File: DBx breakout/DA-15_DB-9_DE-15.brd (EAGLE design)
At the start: 19.1 x 38.1 mm, 3 parts

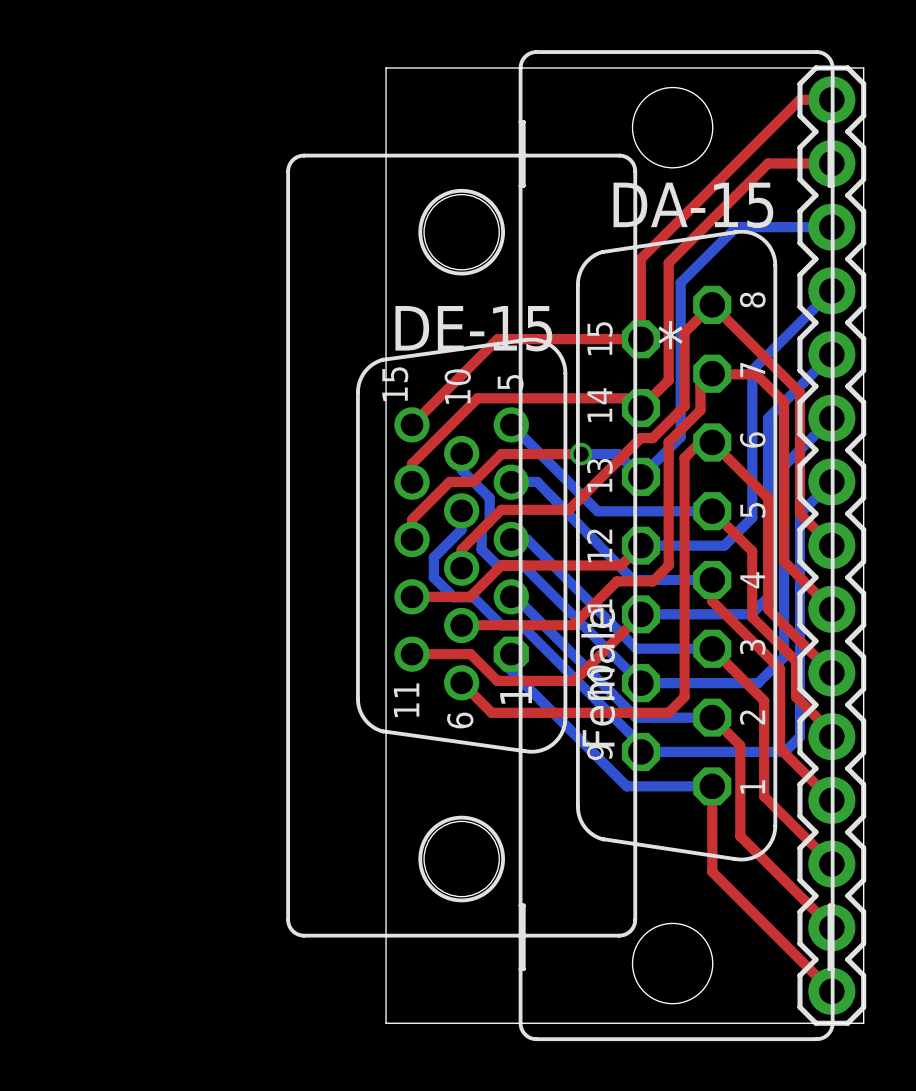
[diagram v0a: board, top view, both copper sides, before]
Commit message: updated board
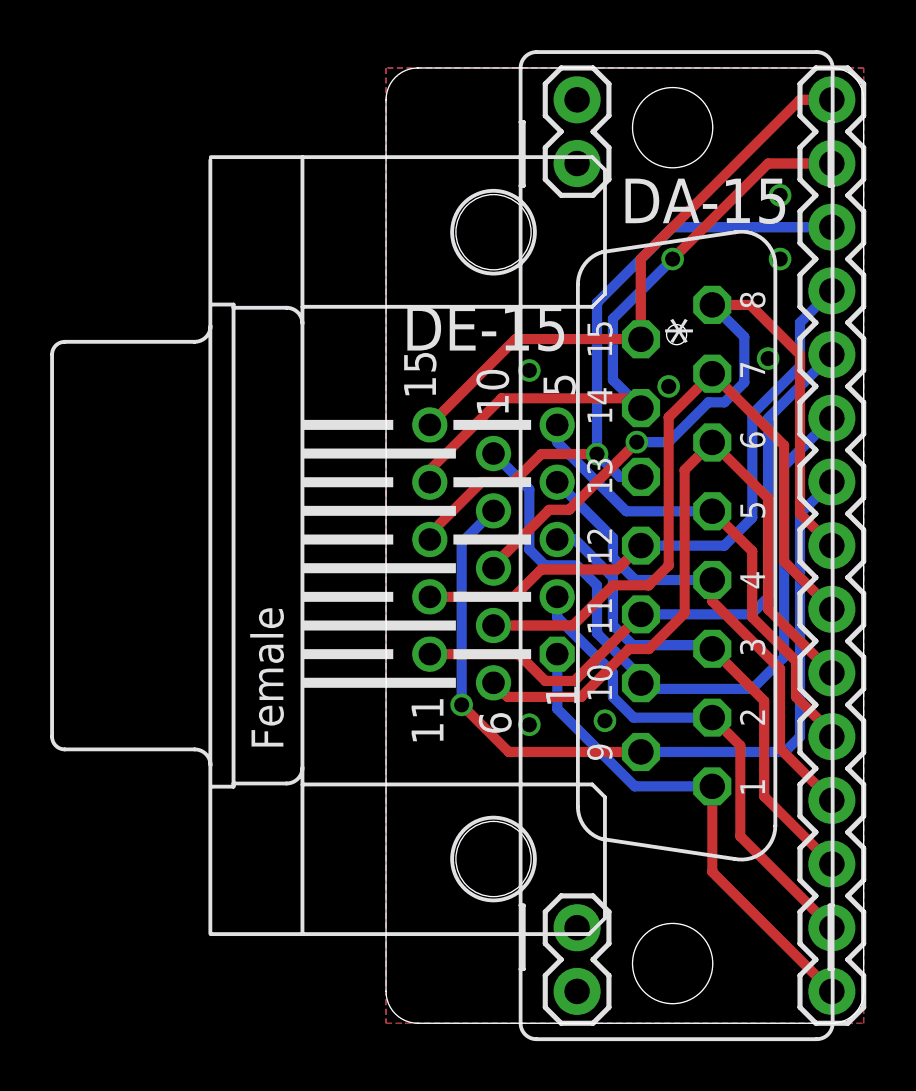
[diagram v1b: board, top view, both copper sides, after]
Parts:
- added RAIL1, RAIL2: (no value), SparkFun-Connectors:1X02
- DE-15: device adafruit:HDF15V -> con-subd:HDF15H
- moved DE-15 1.27 mm to (4.29, 19.1)
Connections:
- new net SHIELD: RAIL1.1, RAIL1.2, RAIL2.1, RAIL2.2
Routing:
- net 6: track 31.7 -> 27.7 mm
- net 7: track 30.0 -> 27.7 mm
- net 9: track 31.7 -> 33.5 mm, vias 0 -> 1
- net 5: track 20.4 -> 19.0 mm
- net 4: track 20.4 -> 19.0 mm
- net 8: track 28.1 -> 29.2 mm, vias 0 -> 1
- net 1: track 20.7 -> 19.8 mm
- net 2: track 20.4 -> 19.6 mm
- net 3: track 20.4 -> 19.7 mm
- net 15: track 24.0 -> 23.3 mm
- net 11: track 26.8 -> 26.1 mm
- net 12: track 25.2 -> 24.5 mm
- net 14: track 25.5 -> 25.6 mm, vias 0 -> 1
- added copper zone on layer 1, net SHIELD
- added copper zone on layer 16, net SHIELD
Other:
- outline, holes or cut-outs redrawn
